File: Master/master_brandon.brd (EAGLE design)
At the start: 84.3 x 69.3 mm, 58 parts, among them J1 ISP, K1 653002114822, K2 653002114822, K3 653002114822, K4 653002114822, U1 ATMEGA128RFA1, U3 ULN2003ANE4, Y1 16MHz, Y2 32.768kHz

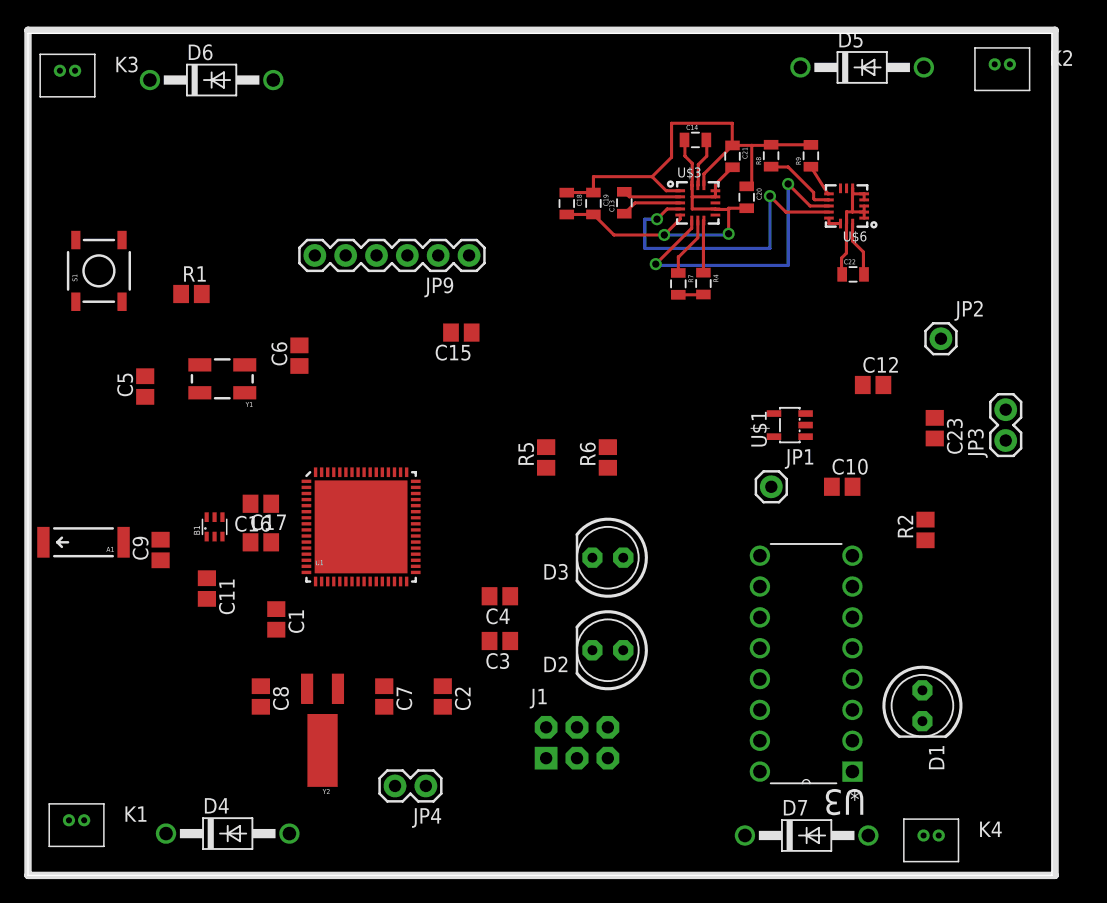
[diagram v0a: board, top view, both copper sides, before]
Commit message: worked on my layout.  The rest can be auto-routed
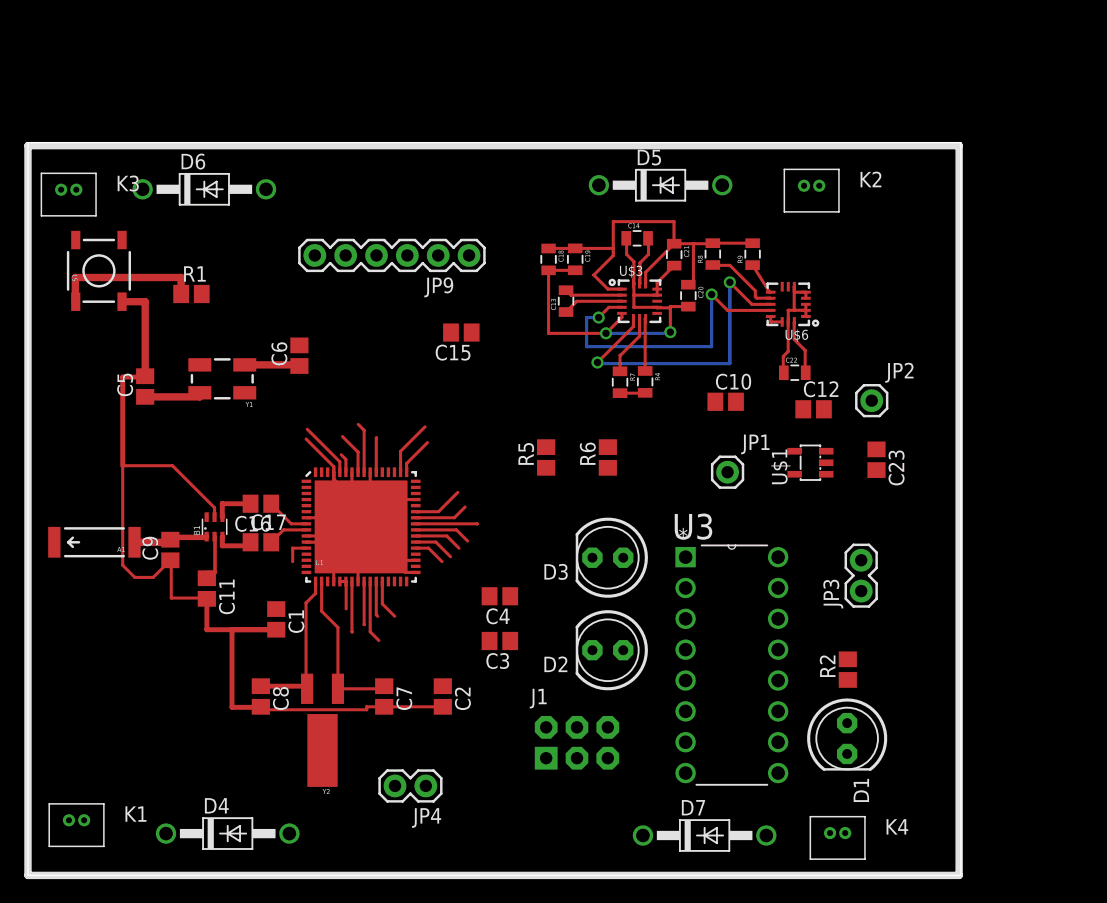
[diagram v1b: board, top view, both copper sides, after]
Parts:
- moved D5 19.2 mm to (52.1, 54.3)
- moved K2 18.6 mm to (64.5, 54.3)
- moved U3 18.0 mm to (61.8, 5.89), turned to 0 degrees
- moved JP3 17.2 mm to (68.6, 20.9)
- moved R2 13.2 mm to (67.5, 14.4)
- moved C10 11.9 mm to (57.5, 36.5)
- moved K3 9.80 mm to (3.35, 53.9)
- moved R4 9.42 mm to (50.8, 38.1)
- moved R9 9.42 mm to (59.7, 48.6)
- moved U$6 9.42 mm to (62.6, 44.5)
- moved C14 9.42 mm to (50.2, 49.9)
- moved C20 9.42 mm to (54.4, 45.2)
- moved R7 9.42 mm to (48.8, 38.1)
- moved R8 9.42 mm to (56.4, 48.6)
- moved U$3 9.42 mm to (50.4, 44.7)
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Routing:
- net GND: track 45.5 -> 177.0 mm
- net RESET: track 0.00 -> 14.4 mm
- net N$5: track 0.00 -> 13.4 mm
- net N$6: track 0.00 -> 13.2 mm
- net N$4: track 0.00 -> 8.73 mm
- net N$3: track 0.00 -> 8.30 mm
- net RFANT: track 0.00 -> 6.27 mm
- net 3.3V: track 41.1 -> 46.7 mm
- net SDA: track 26.6 -> 31.8 mm
- net PB5: track 0.00 -> 5.07 mm
- net AVDD: track 0.00 -> 4.65 mm
- net PB4: track 0.00 -> 4.65 mm
- net PE4: track 0.00 -> 4.57 mm
- net PB6: track 0.00 -> 4.44 mm
- net N$7: track 0.00 -> 4.13 mm
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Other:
- board size 84.3 x 69.3 mm -> 76.8 x 60.3 mm
